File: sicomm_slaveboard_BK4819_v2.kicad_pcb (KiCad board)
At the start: 4 copper layers, 72.4 x 52.2 mm, 127 parts, among them U1 MMZ1005B601CT000, U19 TPLP5907MFX-3.3, U2 MMZ1005B601CT000, U23 CMX994E1, U39 MMZ1005B601CT000, U4 MGA-68563, U44 RFSW8000TR7, X2 26MHz

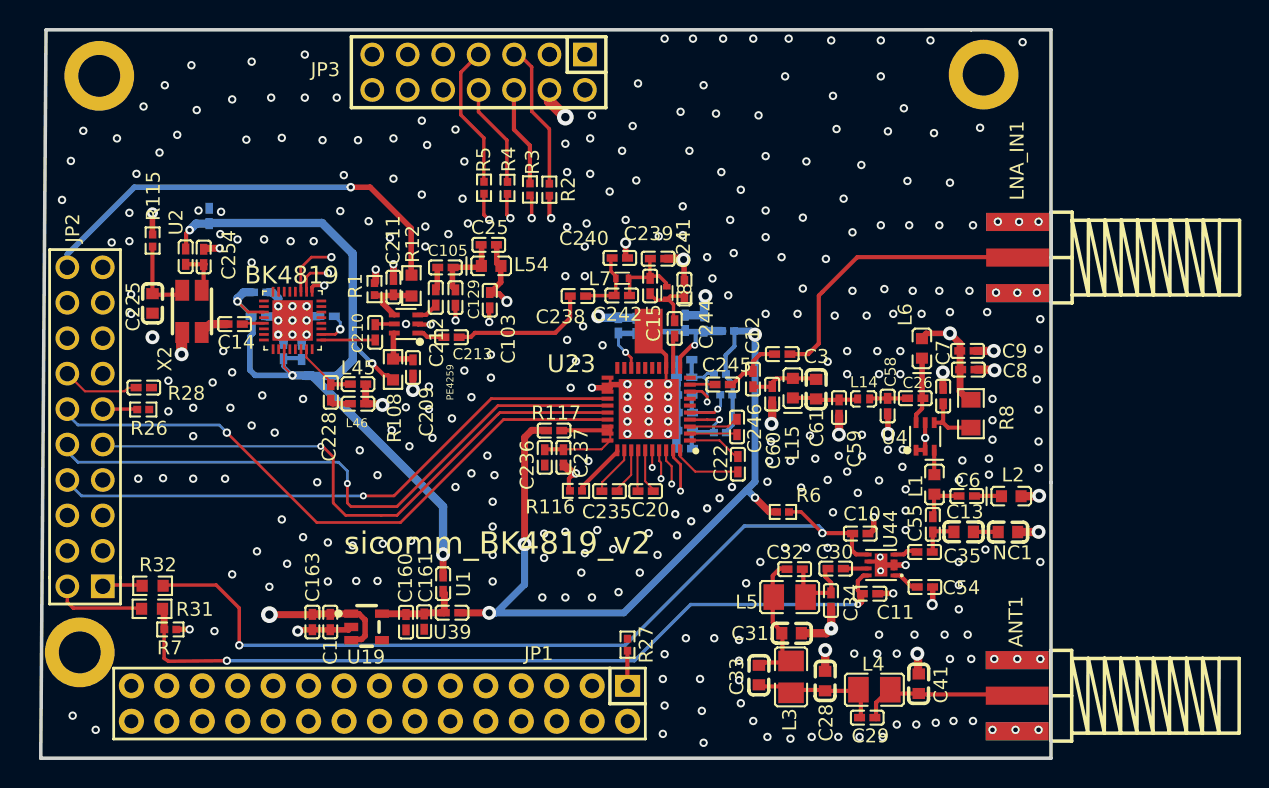
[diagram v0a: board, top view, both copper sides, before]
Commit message: sec
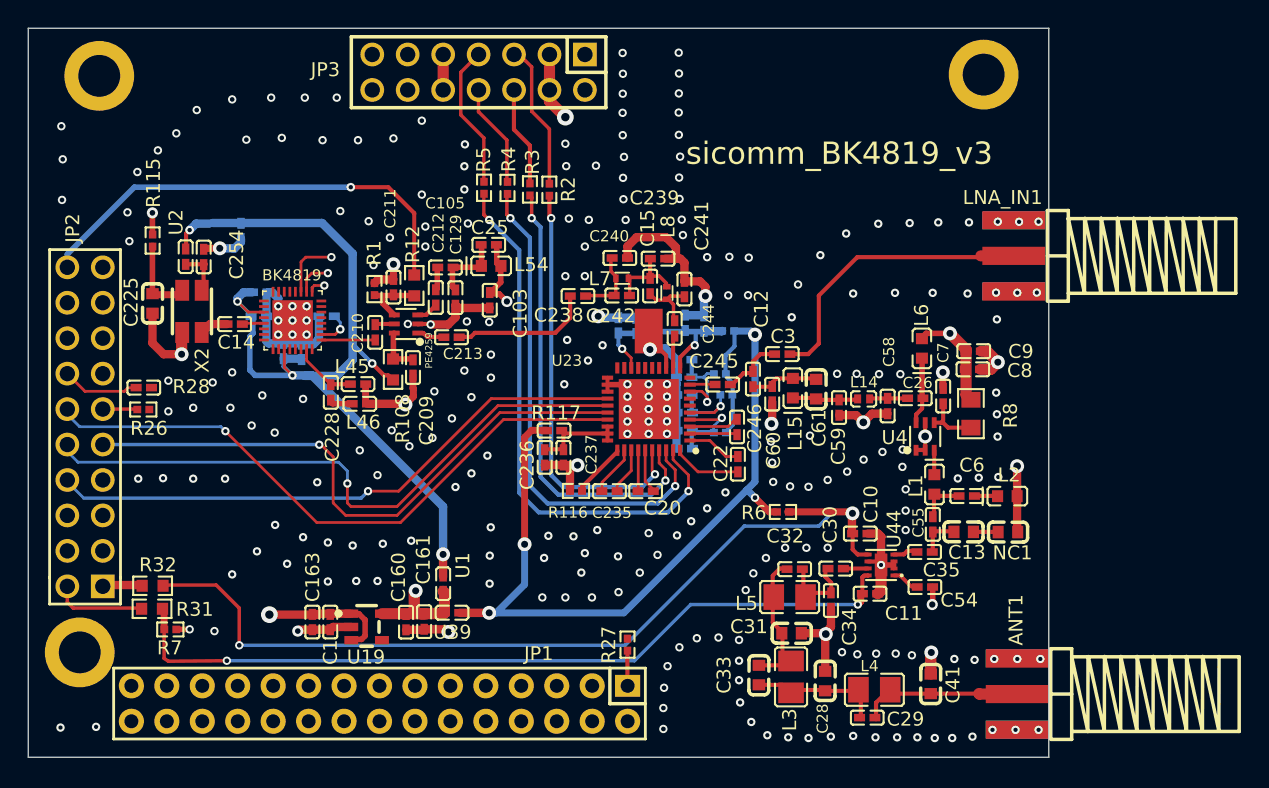
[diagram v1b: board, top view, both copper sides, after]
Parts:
- L46: footprint sicomm_slaveboard_BK4819_v2:L0402 -> easyeda2kicad_foorprint:L0402
- moved C223 2.52 mm to (123.9, 97.6), turned to 90 degrees
- moved C41 0.86 mm to (173.4, 130.1)
- moved C9 0.45 mm to (176.4, 106.2)
- moved C8 0.33 mm to (176.4, 107.5)
- moved LNA_IN1 0.30 mm to (179.3, 99.4)
- moved L2 0.28 mm to (178.8, 116.6)
- moved R12 0.20 mm to (136.3, 101.5)
- moved L46 0.13 mm to (132.4, 110.0)
- moved ANT1 0.12 mm to (179.6, 130.8)
- turned R27 to -90 degrees
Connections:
- L46 pad 2: C228_2 -> Net-(C228-Pad2)
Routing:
- net GND: track 84.6 -> 121.7 mm, vias 363 -> 266
- net Net-(U44-VRF2): track 62.4 -> 65.3 mm
- net Net-(U23-DVDD): track 9.95 -> 7.35 mm
- net A3V3: track 6.02 -> 8.00 mm, vias 0 -> 1
- net Net-(C228-Pad2): track 0.00 -> 1.58 mm
- net C228_2: track 1.58 -> 0.00 mm
- net PE4259_CTL_LMX_CE: track 32.1 -> 33.2 mm
- net Net-(U23-RXIN): track 38.6 -> 39.4 mm
- net Net-(C28-Pad2): track 9.43 -> 10.2 mm
- net Net-(U23-RXQN): track 32.4 -> 32.9 mm
- net VBAT: track 24.4 -> 23.9 mm, vias 2 -> 1
- net VCC_LO: vias 3 -> 2
- net Net-(PE4259-CTRL): vias 1 -> 0
- added copper zone on In2.Cu, net A3V3
- removed copper zone on In2.Cu, net GND
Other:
- board size 72.4 x 52.2 mm -> 73.1 x 52.2 mm
- board text added: "26/11/2024"
- board text added: "sicomm_BK4819_v3"
- board text removed: "14/11/2024"
- board text removed: "sicomm_BK4819_v2"
